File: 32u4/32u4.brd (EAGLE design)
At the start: 35.6 x 29.8 mm, 16 parts, among them J1 AVR_SPI_PRG_62X3_LOCK

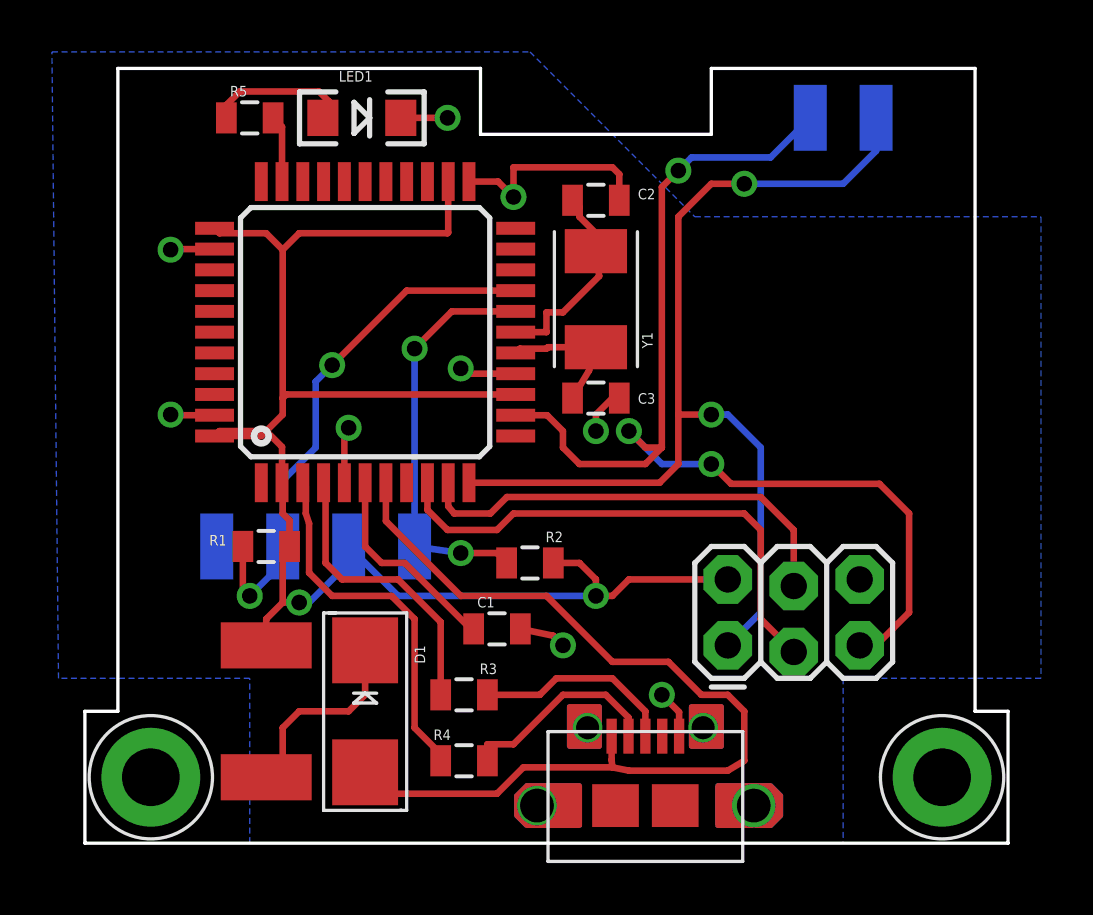
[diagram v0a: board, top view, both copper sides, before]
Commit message: Latest controller revision
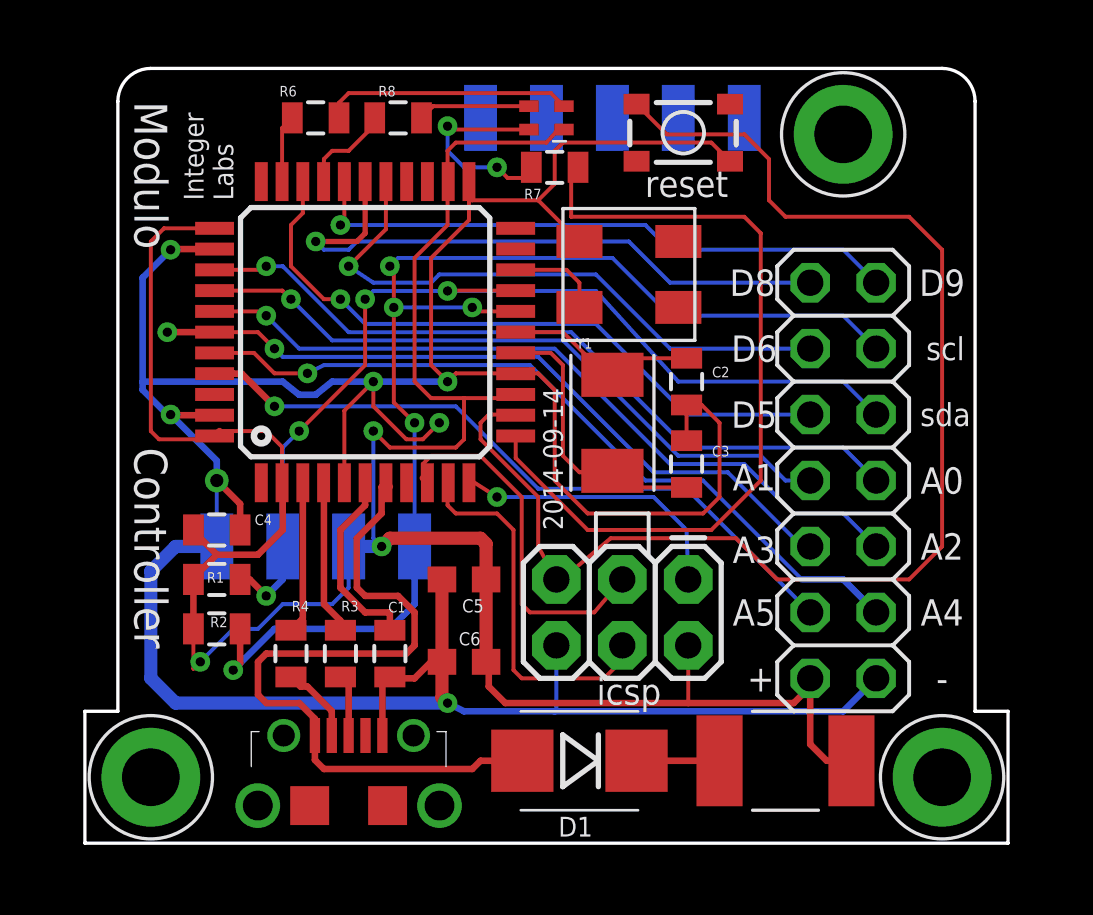
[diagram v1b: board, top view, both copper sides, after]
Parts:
- removed LED1: (no value), SparkFun-LED:LED-1206
- removed R5: (no value), SparkFun-Resistors:0805
- added C4: 1uF, SparkFun-Capacitors:0805
- added C5, C6: 100uF, resistor:C1608
- added JP2: (no value), pinhead:2X07
- added R6, R7: 150, SparkFun-Resistors:0805
- added R8: 330, SparkFun-Resistors:0805
- added S1: SWITCH-MOMENTARY-2SMD-3, SparkFun-Electromechanical:TACTILE_SWITCH_SMD-3
- added U$5: LED-RGB, IntegerLabs:LED-LITEON-SMD-RGB
- added U$6: TACT-SWITCHBOURNS-7914J, IntegerLabs:BOURNS-7914J
- C2, C3: value (none) -> 18pF
- D1: value (none) -> b340b; device adafruit:SMADIODE -> SparkFun-DiscreteSemi:SMB-DIODE
- J1: value AVR_SPI_PRG_62X3_LOCK -> AVR_SPI_PRG_6PTH; device SparkFun-Connectors:2X3_LOCK -> SparkFun-Connectors:2X3
- R1, R2: value (none) -> 2k
- U$4: value USB-MICRO-AB -> USBFCI-MICROB; device IntegerLabs:MOLEX-MICROAB -> IntegerLabs:USB-MICROB-FCI
- moved U$1 20.1 mm to (27.0, 3.17), turned to 180 degrees
- moved R2 12.3 mm to (5.08, 8.26), turned to 0 degrees
- moved U$4 11.4 mm to (10.2, 1.45)
- moved D1 8.47 mm to (19.1, 3.17), turned to 180 degrees
- moved R4 7.84 mm to (7.94, 7.30), turned to 90 degrees
- moved C2 7.81 mm to (23.2, 17.8), turned to 90 degrees
- moved R3 5.02 mm to (9.84, 7.30), turned to 90 degrees
- moved Y1 4.80 mm to (20.3, 16.2)
- moved C3 4.32 mm to (23.2, 14.6), turned to 270 degrees
- moved C1 4.24 mm to (11.7, 7.30), turned to 270 degrees
- moved J1 2.96 mm to (23.2, 10.2), turned to 180 degrees
- moved R1 2.29 mm to (5.08, 10.2), turned to 0 degrees
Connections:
- removed net LED: R5.2, U$2.32
- removed net N$3: LED1.A, R5.1
- new net A0: JP2.7, U$2.36
- new net A1: JP2.8, U$2.37
- new net A2: JP2.5, U$2.38
- new net A3: JP2.6, U$2.39
- new net A4: JP2.3, U$2.40
- new net A5: JP2.4, U$2.41
- new net B: R6.1, U$2.32
- new net D5: JP2.10, U$2.31
- new net D6: JP2.12, U$2.27
- new net D8: JP2.14, U$2.28
- new net D9: JP2.13, U$2.29
- new net G: R7.1, U$2.12
- new net N$10: R6.2, U$5.1
- new net N$6: R8.2, U$5.2
- new net N$7: R7.2, U$5.3
- new net R: R8.1, U$2.30
- new net SWITCH: U$2.20, U$6.POS$1
- net D+: now also U$4.P3; no longer U$4.3
- net D-: now also U$4.P2; no longer U$4.2
- net GND: now also C4.2, C5.2, C6.2, JP2.1, S1.1, U$3.BUS0, U$4.P5, U$6.NEG$1; no longer LED1.C, U$3.GND, U$4.5
- net MISO: no longer U$3.MISO
- net RESET: now also S1.4; no longer U$3.RESET
- net SCL: now also JP2.11, U$3.BUS3; no longer U$3.SCL
- net SDA: now also JP2.9, U$3.BUS1; no longer U$3.SDA
- net VBUS: now also U$4.P1; no longer U$4.1
- net VCC: now also C4.1, C5.1, C6.1, JP2.2, U$3.BUS2, U$5.4; no longer U$3.VCC
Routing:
- net GND: track 23.4 -> 132.2 mm, vias 9 -> 7
- net VCC: track 63.4 -> 97.1 mm, vias 2 -> 3
- net SCL: track 15.8 -> 48.2 mm, vias 2 -> 5
- net G: track 0.00 -> 31.4 mm
- net A4: track 0.00 -> 29.8 mm, vias 0 -> 1
- net A2: track 0.00 -> 29.2 mm, vias 0 -> 1
- net A0: track 0.00 -> 29.0 mm, vias 0 -> 1
- net MISO: track 39.7 -> 11.1 mm, vias 2 -> 1
- net A3: track 0.00 -> 28.2 mm, vias 0 -> 2
- net A5: track 0.00 -> 26.8 mm, vias 0 -> 1
- net A1: track 0.00 -> 26.0 mm, vias 0 -> 1
- net D5: track 0.00 -> 25.8 mm, vias 0 -> 1
- net D8: track 0.00 -> 24.0 mm, vias 0 -> 1
- net D9: track 0.00 -> 23.3 mm, vias 0 -> 1
- net D6: track 0.00 -> 23.1 mm, vias 0 -> 1
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- removed copper zone on layer 16, net GND
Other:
- outline, holes or cut-outs redrawn
- board text added: "+"
- board text added: "-"
- board text added: "2014-09-14"
- board text added: "A0"
- board text added: "A1"
- board text added: "A2"
- board text added: "A3"
- board text added: "A4"
- board text added: "A5"
- board text added: "Controller"
- board text added: "D5"
- board text added: "D6"
- board text added: "D8"
- board text added: "D9"
- board text added: "Integer Labs"
- board text added: "Modulo"
- board text added: "icsp"
- board text added: "reset"
- board text added: "scl"
- board text added: "sda"
